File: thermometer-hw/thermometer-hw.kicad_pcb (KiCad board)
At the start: 2 copper layers, 30.2 x 46.5 mm, 16 parts, among them J1 Conn_01x03_Pin, J2 PWR, J3 ICSP, U1 ATtiny24A-SS, U2 MAX7221xWG, U3 CC56-12SRWA

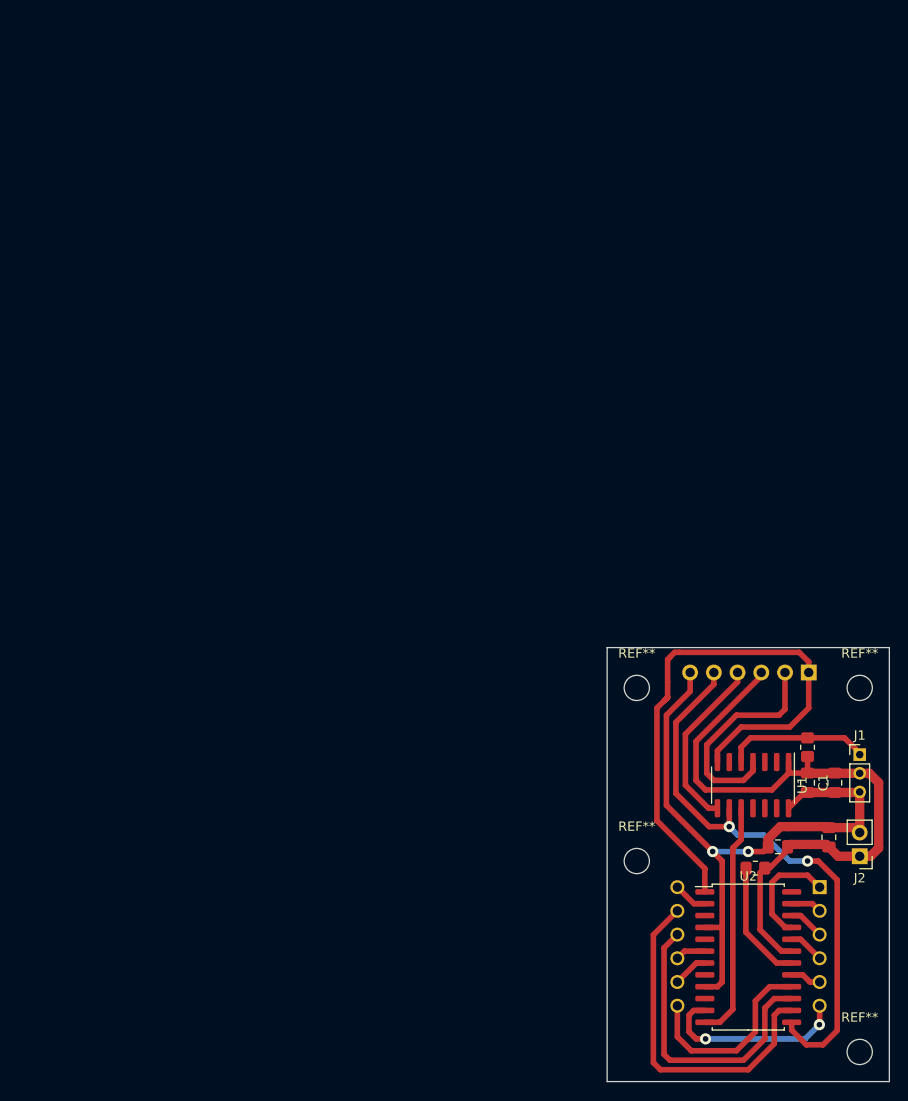
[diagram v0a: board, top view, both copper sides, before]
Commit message: Firmware progress
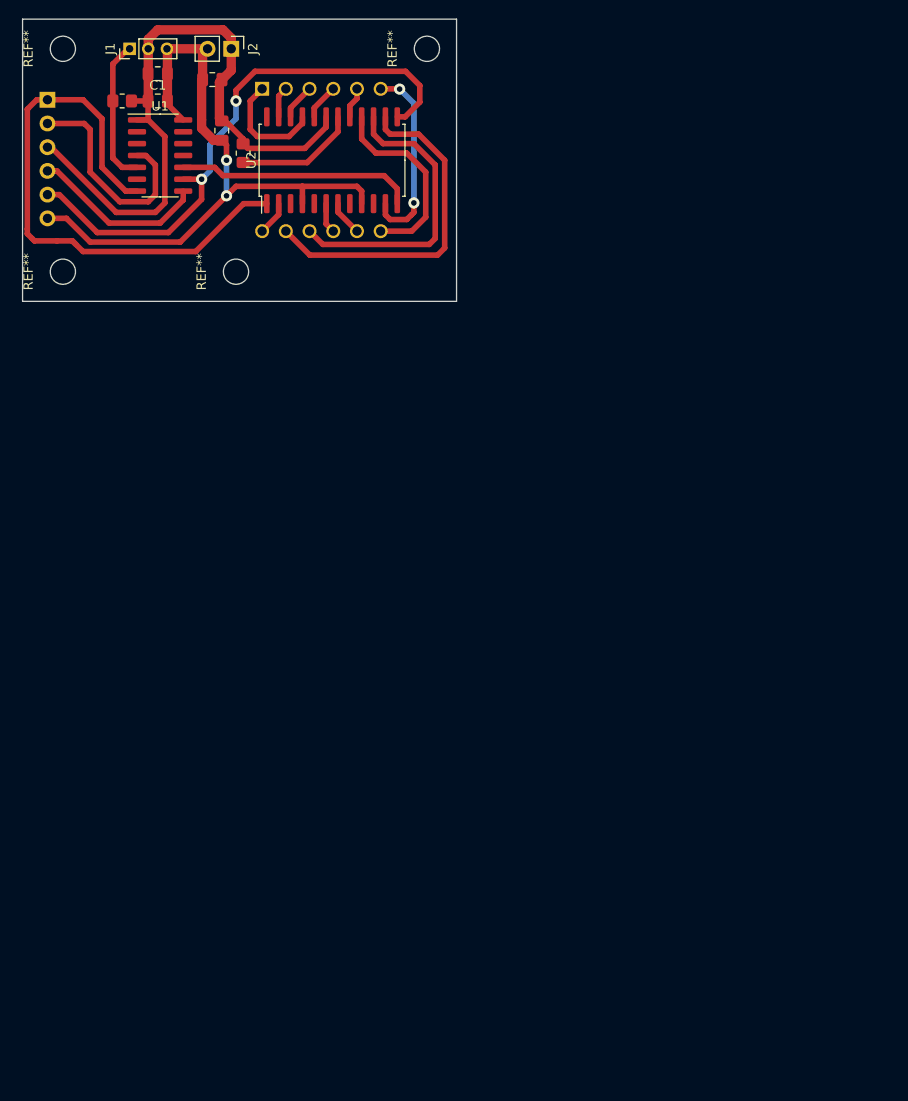
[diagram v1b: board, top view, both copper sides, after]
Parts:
- moved REF** 117.0 mm to (43.8, -28.1), turned to 90 degrees
- moved J2 109.6 mm to (22.9, -28.1), turned to -90 degrees
- moved REF** 109.4 mm to (4.83, -28.1), turned to 90 degrees
- moved J1 108.8 mm to (12.0, -28.1), turned to 90 degrees
- moved C3 105.0 mm to (15.0, -25.4), turned to 0 degrees
- moved C4 104.6 mm to (20.8, -24.8), turned to 180 degrees
- moved U3 104.3 mm to (26.2, -23.8), turned to -90 degrees
- moved J3 102.0 mm to (3.17, -22.6), turned to 180 degrees
- moved R2 100.9 mm to (11.2, -22.5), turned to 180 degrees
- moved C1 100.9 mm to (15.0, -22.5), turned to 0 degrees
- moved C2 97.1 mm to (21.8, -19.3), turned to -90 degrees
- moved U2 96.3 mm to (33.7, -16.1), turned to 90 degrees
- moved R1 94.2 mm to (24.1, -16.9), turned to -90 degrees
- moved U1 92.6 mm to (15.2, -16.6), turned to 0 degrees
- moved REF** 76.3 mm to (23.4, -4.19), turned to 90 degrees
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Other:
- board size 30.2 x 46.5 mm -> 46.5 x 30.2 mm
